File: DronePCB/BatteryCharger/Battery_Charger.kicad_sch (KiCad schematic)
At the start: 43 parts, among them Q1 AO3400A, Q2 AO3400A, Q3 SiS454DN, Q4 SiS454DN, Q5 AO3400A, U1 BQ24725A

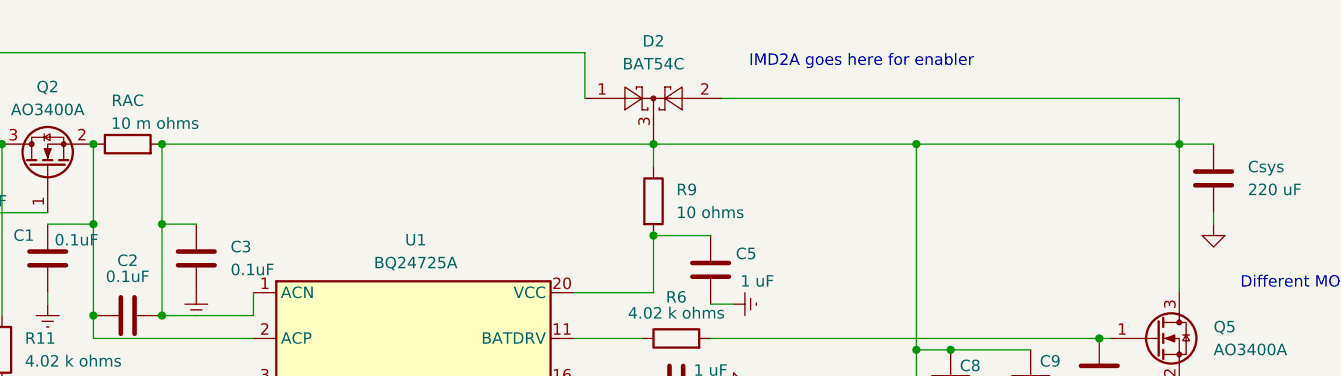
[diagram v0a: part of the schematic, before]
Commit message: Add files via upload
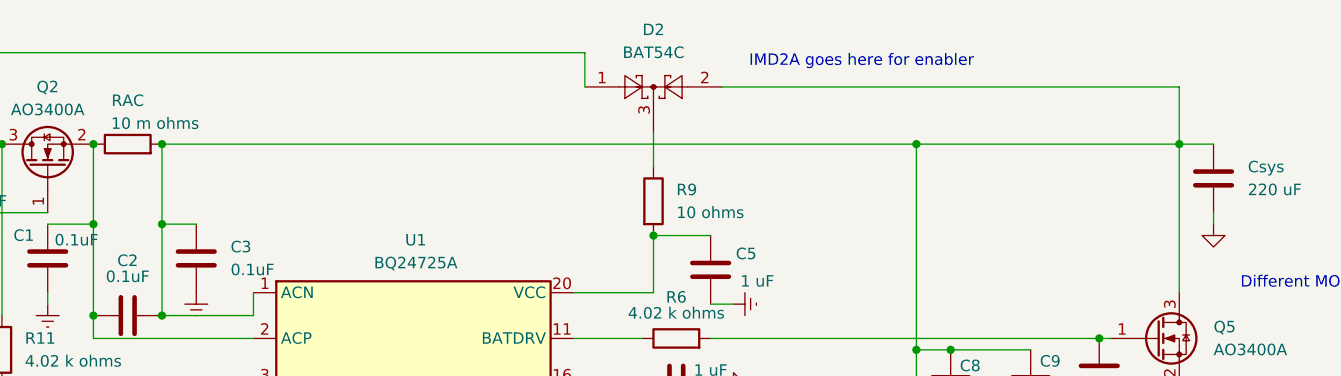
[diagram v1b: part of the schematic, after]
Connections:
- net at C2.1, C3.1, C8.1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: no longer D2.3, R9.1
- new net: D2.3, R9.1
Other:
- moved on the sheet: D2
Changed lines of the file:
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@@
 	)
 	(junction
-		(at 128.27 26.67)
-		(diameter 0)
-		(color 0 0 0 0)
-	)
-	(junction
 		(at 124.46 68.58)
 		(diameter 0)
@@
 	(wire
 		(pts
-			(xy 135.89 21.59) (xy 186.69 21.59)
+			(xy 135.89 20.32) (xy 186.69 20.32)
 		)
 		(stroke
@@
 	(wire
 		(pts
-			(xy 186.69 21.59) (xy 186.69 26.67)
+			(xy 186.69 20.32) (xy 186.69 26.67)
 		)
 		(stroke
@@
 	(wire
 		(pts
-			(xy 128.27 26.67) (xy 73.66 26.67)
-		)
-		(stroke
-			(width 0)
-			(type default)
-		)
-	)
-	(wire
-		(pts
 			(xy 144.78 82.55) (xy 135.89 82.55)
 		)
@@
 	(wire
 		(pts
-			(xy 120.65 21.59) (xy 120.65 16.51)
+			(xy 120.65 20.32) (xy 120.65 16.51)
 		)
 		(stroke
@@
 	(wire
 		(pts
-			(xy 128.27 26.67) (xy 128.27 29.21)
+			(xy 157.48 49.53) (xy 157.48 26.67)
 		)
 		(stroke
@@
 	(wire
 		(pts
-			(xy 157.48 49.53) (xy 157.48 26.67)
+			(xy 71.12 86.36) (xy 49.53 86.36)
 		)
 		(stroke
@@
 	(wire
 		(pts
-			(xy 71.12 86.36) (xy 49.53 86.36)
+			(xy 25.4 63.5) (xy 25.4 64.77)
 		)
 		(stroke
@@
 	(wire
 		(pts
-			(xy 25.4 63.5) (xy 25.4 64.77)
+			(xy 83.82 58.42) (xy 41.91 58.42)
 		)
 		(stroke
@@
 	(wire
 		(pts
-			(xy 83.82 58.42) (xy 41.91 58.42)
+			(xy 186.69 58.42) (xy 186.69 90.17)
 		)
 		(stroke
@@
 	(wire
 		(pts
-			(xy 186.69 58.42) (xy 186.69 90.17)
+			(xy 78.74 96.52) (xy 78.74 97.79)
 		)
 		(stroke
@@
 	(wire
 		(pts
-			(xy 78.74 96.52) (xy 78.74 97.79)
+			(xy 128.27 25.4) (xy 128.27 29.21)
 		)
 		(stroke
@@
 	(wire
 		(pts
+			(xy 73.66 26.67) (xy 157.48 26.67)
+		)
+		(stroke
+			(width 0)
+			(type default)
+		)
+	)
+	(wire
+		(pts
 			(xy 186.69 53.34) (xy 186.69 58.42)
 		)
@@
 		)
 	)
-	(wire
-		(pts
-			(xy 157.48 26.67) (xy 128.27 26.67)
-		)
-		(stroke
-			(width 0)
-			(type default)
-		)
-	)
 	(symbol
 		(lib_id "Device:R")
@@
 	(symbol
 		(lib_id "Diode:BAT54C")
-		(at 128.27 21.59 0)
+		(at 128.27 20.32 0)
 		(unit 1)
 		(body_style 1)
@@
 		(fields_autoplaced yes)
 		(property "Reference" "D2"
-			(at 128.27 15.24 0)
+			(at 128.27 13.97 0)
 			(show_name no)
 			(do_not_autoplace no)
@@
 		)
 		(property "Value" "BAT54C"
-			(at 128.27 17.78 0)
+			(at 128.27 16.51 0)
 			(show_name no)
 			(do_not_autoplace no)
@@
 		)
 		(property "Footprint" "Package_TO_SOT_SMD:SOT-23"
-			(at 130.175 18.415 0)
+			(at 130.175 17.145 0)
 			(hide yes)
 			(show_name no)
@@
 		)
 		(property "Datasheet" "http://www.diodes.com/_files/datasheets/ds11005.pdf"
-			(at 126.238 21.59 0)
+			(at 126.238 20.32 0)
 			(hide yes)
 			(show_name no)
@@
 		)
 		(property "Description" "dual schottky barrier diode, common cathode"
-			(at 128.27 21.59 0)
+			(at 128.27 20.32 0)
 			(hide yes)
 			(show_name no)
